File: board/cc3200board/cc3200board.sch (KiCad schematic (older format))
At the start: 38 parts, among them U2 N25Q128A13ESE40E, X1 32.768kH, X2 ABM3B-40.000MHZ-10-1-U-T

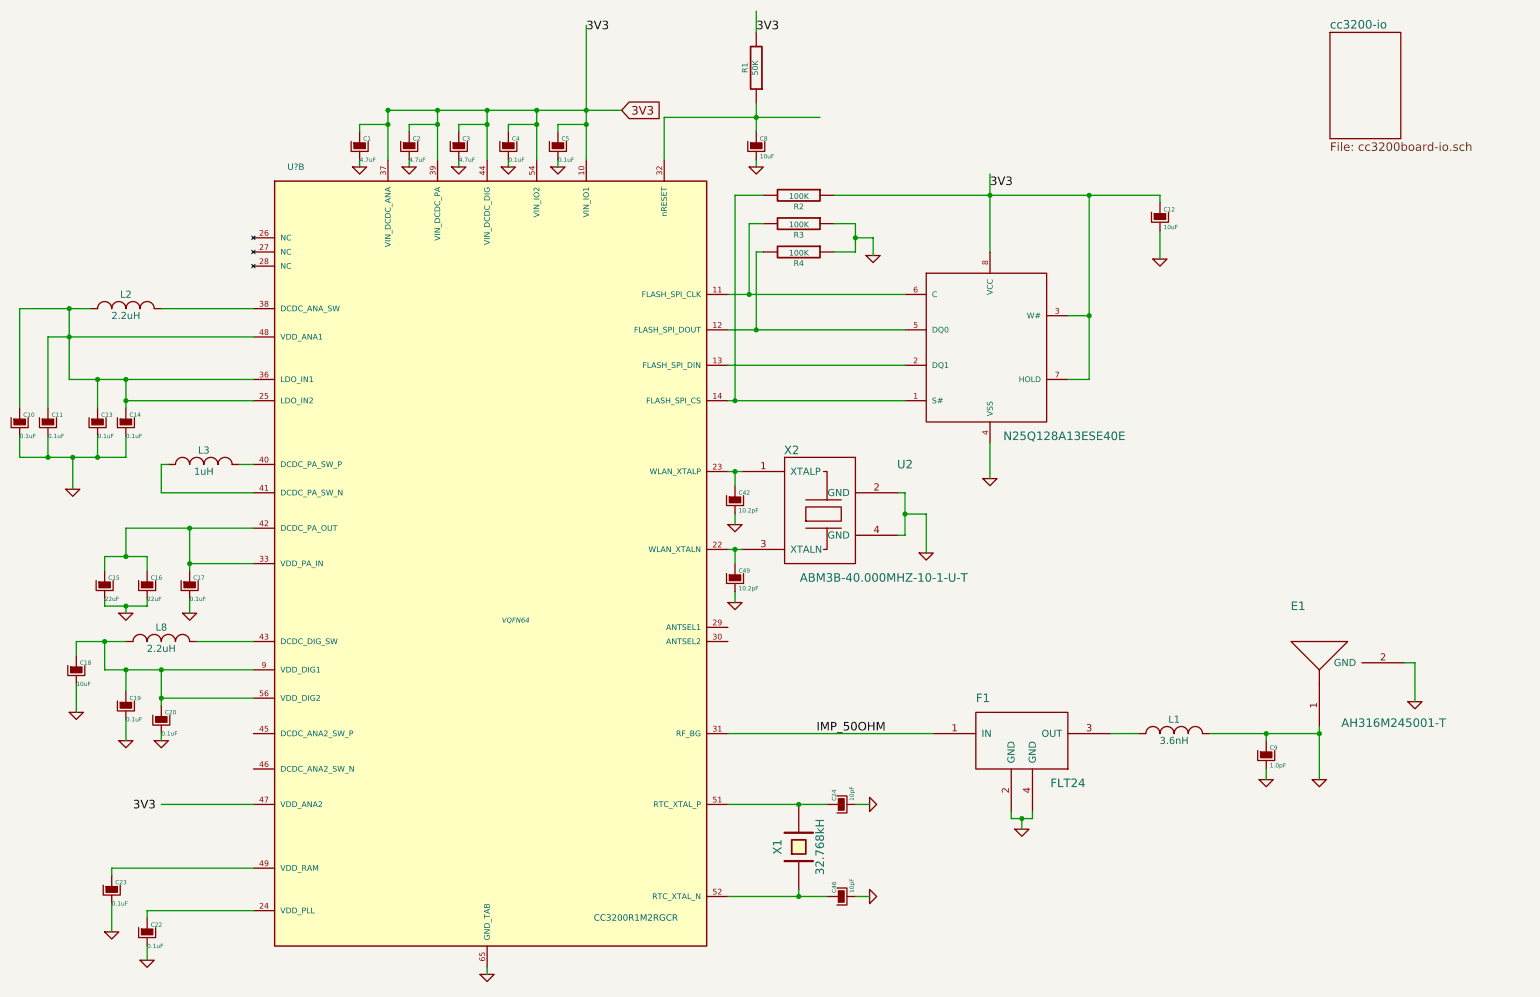
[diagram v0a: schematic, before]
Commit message: Committing final changes
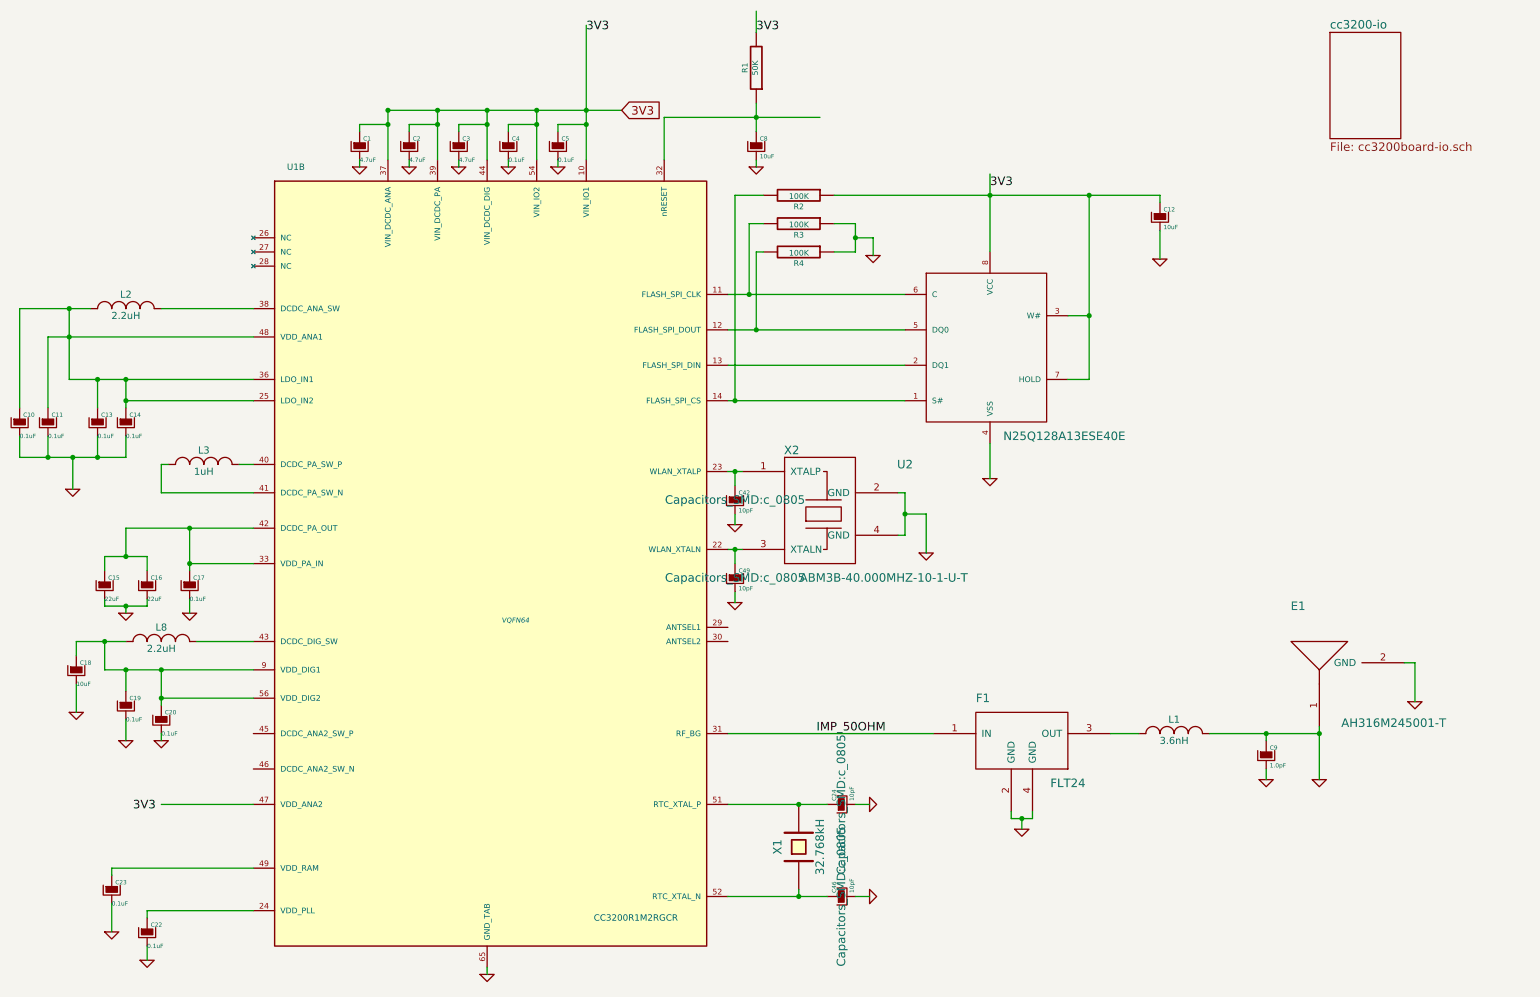
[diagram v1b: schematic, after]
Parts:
- C1, C10, C11, C12, C13, C14, C15, C16, C17, C18, C19, C2, C20, C22, C23, C3, C4, C5, C8, C9, L1, L2, L3, L8, R1, R2, R3, R4, U2, X1: footprint ~ -> (none)
- C24, C46: footprint ~ -> Capacitors_SMD:c_0805
- C42, C49: value 10.2pF -> 10pF; footprint ~ -> Capacitors_SMD:c_0805
- gave numbers to parts that had none: 1
